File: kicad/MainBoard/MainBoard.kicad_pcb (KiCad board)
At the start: 2 copper layers, 191.5 x 166.3 mm, 105 parts, among them J1 CHAN1, J10 ACC Port, J11 433TX, J12 VDC INPUT, J13 BAT, J14 TRG1, J15 TRG2, J16 FP-BUTTONS, J17 EXPAN2, J18 OUTPUT_BOARD_POWER, J19 FrontPanel, J2 CHAN2, J20 I2C, J21 EXPAN3, J3 OUTPUT_BOARD_IO, J4 OUTPUT_BOARD_FP, J5 CHAN4, J6 LCD, J7 CHAN3, J8 EXPAN1, J9 AudioJack3_SwitchTR, SW1 SW_SPST, U1 AT24C04C-PUM, U2 UT232A, U3 LM2941T, U4 Pico, U5 L78L33ACZTR, U6 LM2576T-5, U7 PCF8574, U8 PCF8574

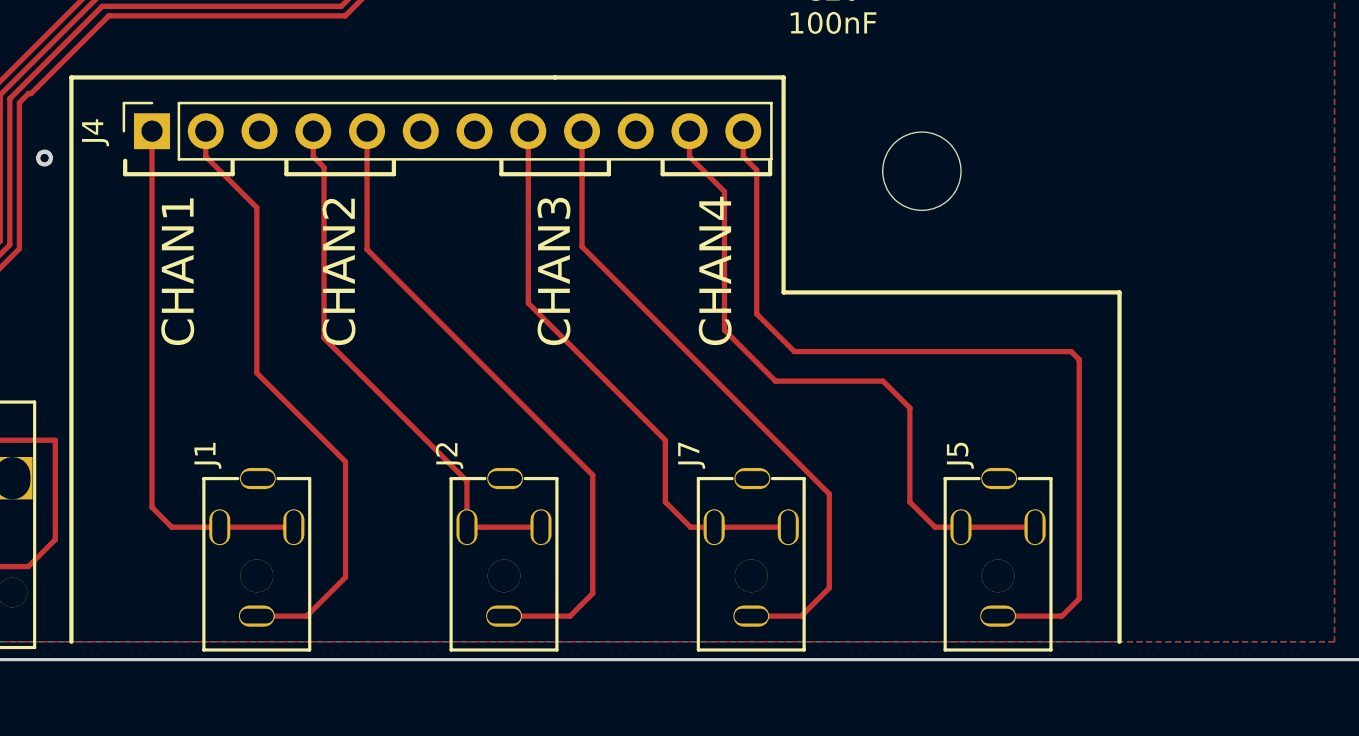
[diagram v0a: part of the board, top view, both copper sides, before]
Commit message: Before 3.5mm footprint switch
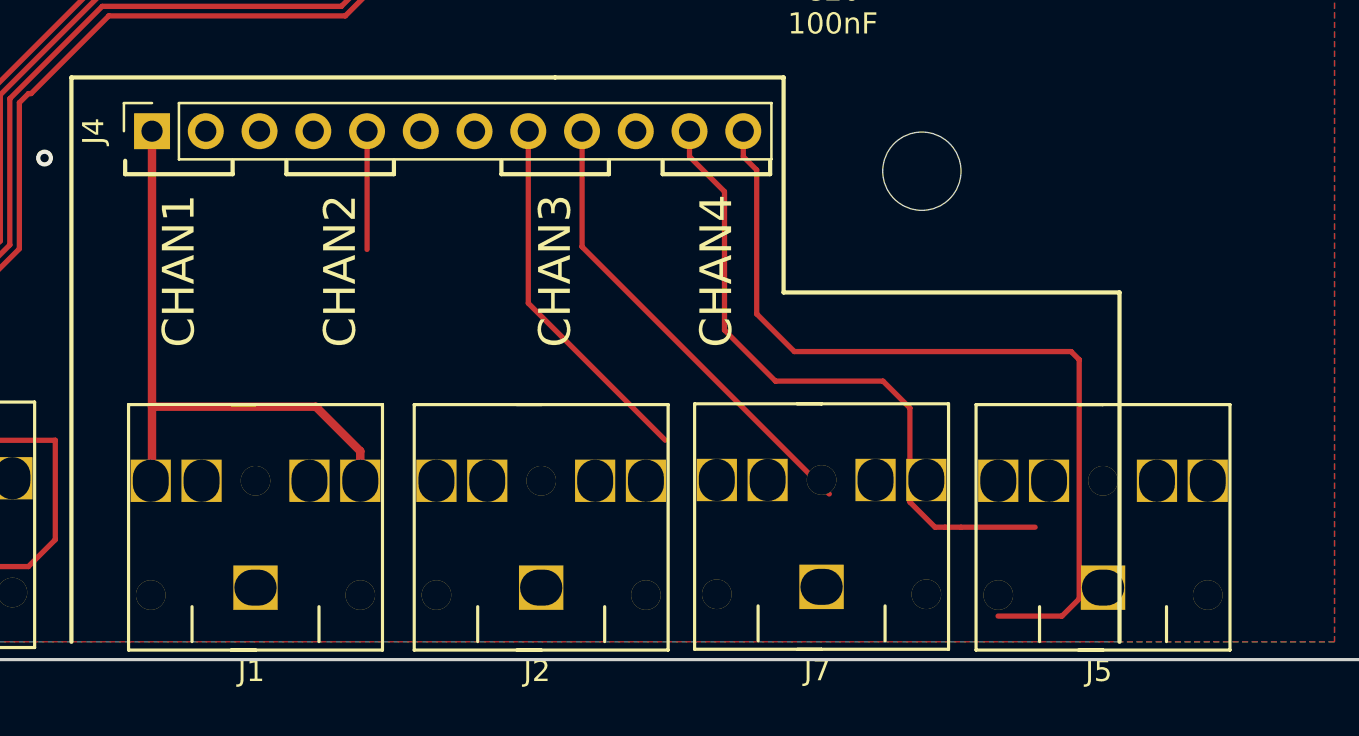
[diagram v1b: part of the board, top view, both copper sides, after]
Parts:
- J1, J5, J7: footprint ProjLib:PJ-2100B-4A -> ProjLib:PJ-3062-CO
- J2: value CHAN2 -> CHAN1; footprint ProjLib:PJ-2100B-4A -> ProjLib:PJ-3062-CO
- moved J5 11.8 mm to (196.9, 183.0), turned to 180 degrees
- moved J7 10.4 mm to (183.7, 183.0), turned to 180 degrees
- moved J2 9.20 mm to (170.4, 183.0), turned to 180 degrees
- moved J1 7.89 mm to (156.9, 183.0), turned to 180 degrees
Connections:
- J1 pad R: unconnected-(J1-PadR) -> Net-(J4-Pin_1)
- J2 pad R: unconnected-(J2-PadR) -> Net-(J4-Pin_4)
- J5 pad R: unconnected-(J5-PadR) -> Net-(J4-Pin_11)
- J7 pad R: unconnected-(J7-PadR) -> Net-(J4-Pin_8)
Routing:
- net Net-(J4-Pin_2): track 28.8 -> 0.00 mm
- net Net-(J4-Pin_5): track 30.9 -> 5.59 mm
- net Net-(J4-Pin_4): track 25.2 -> 0.00 mm
- net Net-(J4-Pin_8): track 26.5 -> 17.3 mm
- net Net-(J4-Pin_9): track 30.7 -> 22.0 mm
- net Net-(J4-Pin_1): track 24.9 -> 28.7 mm
